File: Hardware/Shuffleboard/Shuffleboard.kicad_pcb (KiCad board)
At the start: 4 copper layers, 131 x 132.4 mm, 46 parts, among them IC1 DG3157EDL-T1-GE3, IC2 DG3157EDL-T1-GE3, J1 1869279, J2 1869279, J3 Conn_01x10, Q1 NMOS, U1 COM-09032, U2 PAM8302AAS, U3 LMV331

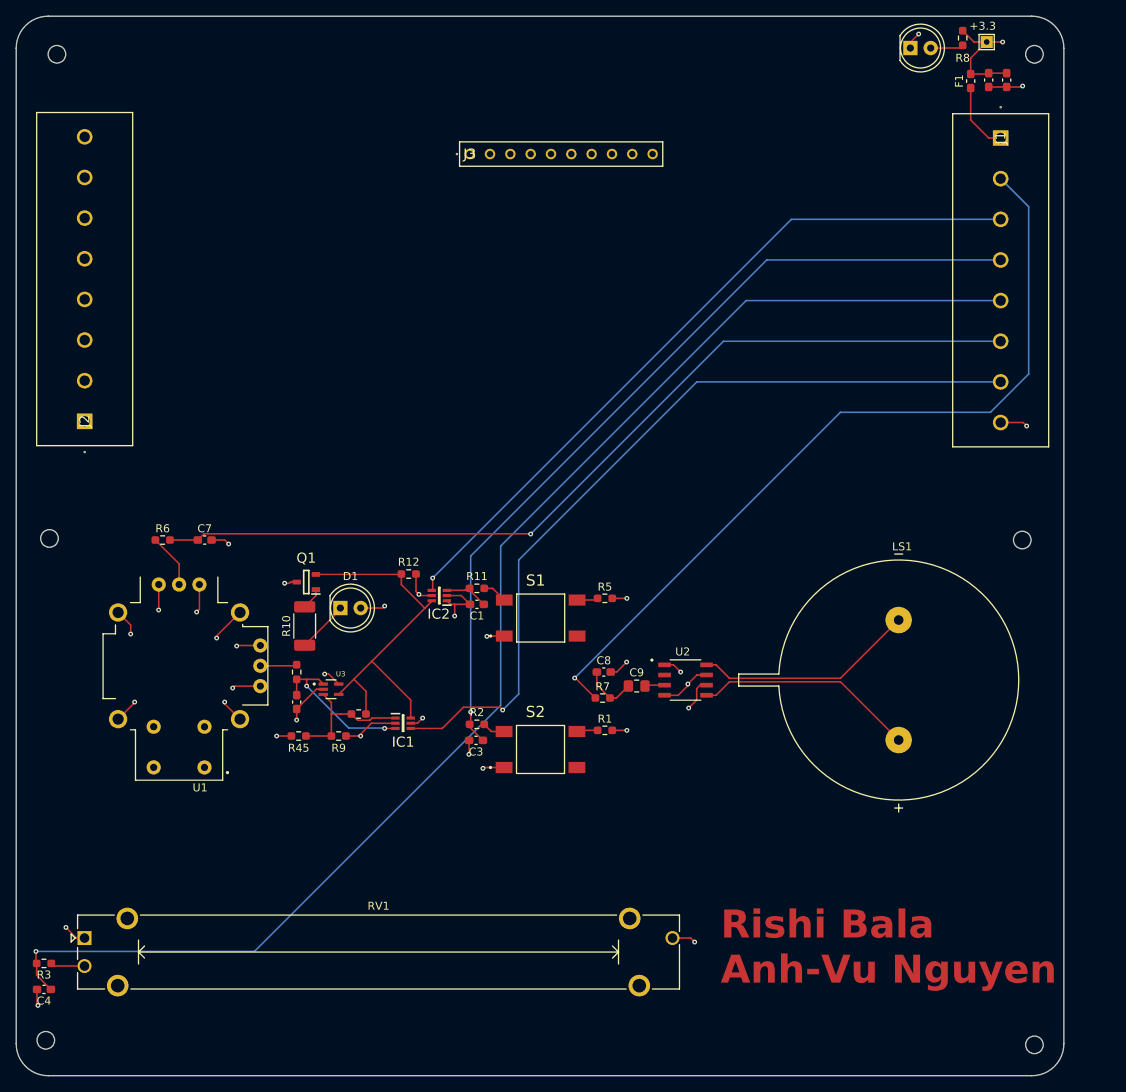
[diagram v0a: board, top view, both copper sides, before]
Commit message: jlc eng fee
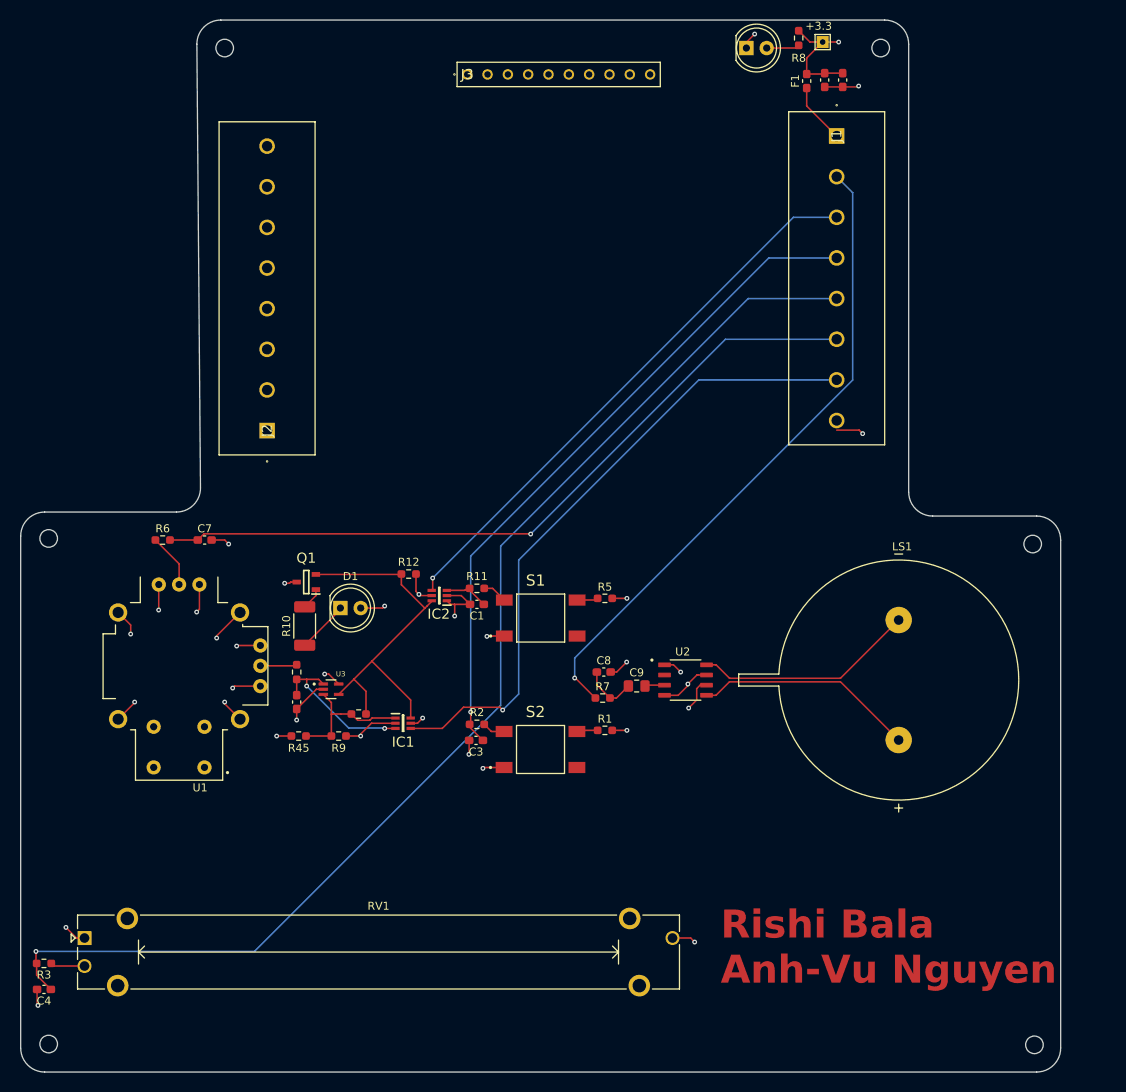
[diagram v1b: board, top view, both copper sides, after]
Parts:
- moved J2 22.8 mm to (140.8, 76.3)
- moved H2 21.0 mm to (135.5, 28.5)
- moved J1 20.5 mm to (212.0, 39.5)
- moved C2 20.5 mm to (210.5, 32.5)
- moved C6 20.5 mm to (212.8, 32.5)
- moved D32 20.5 mm to (200.7, 28.5)
- moved F1 20.5 mm to (208.2, 32.6)
- moved R8 20.5 mm to (207.2, 27.2)
- moved TP2 20.5 mm to (210.2, 27.8)
- moved H3 19.2 mm to (217.5, 28.5)
- moved J3 9.95 mm to (165.8, 31.8)
- moved H5 1.39 mm to (236.5, 90.5)
- moved H1 0.59 mm to (113.5, 153.0)
- moved H6 0.10 mm to (113.5, 89.8)
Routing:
- net /DACOut: track 102.0 -> 81.5 mm
- net /Connector/HOR_PB18_ADC1_5: track 114.2 -> 93.8 mm
- net /PB4SHOOT: track 91.2 -> 70.8 mm
- net /PB1RST: track 105.4 -> 85.0 mm
- net /Connector/POS_PB17_ADC1_4: track 171.5 -> 151.1 mm
- net /Connector/VER_PB19_ADC1_6: track 101.8 -> 81.4 mm
- net /3.3VIN: track 8.68 -> 7.55 mm
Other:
- board size 131 x 132.4 mm -> 130 x 131.5 mm
